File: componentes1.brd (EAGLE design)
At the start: 160 x 100 mm, 14 parts, among them IC1 LD117AS33TR, K1 CQ1-12V, T1 BC337, U1 DS1307Z, X1 32.768KHZ

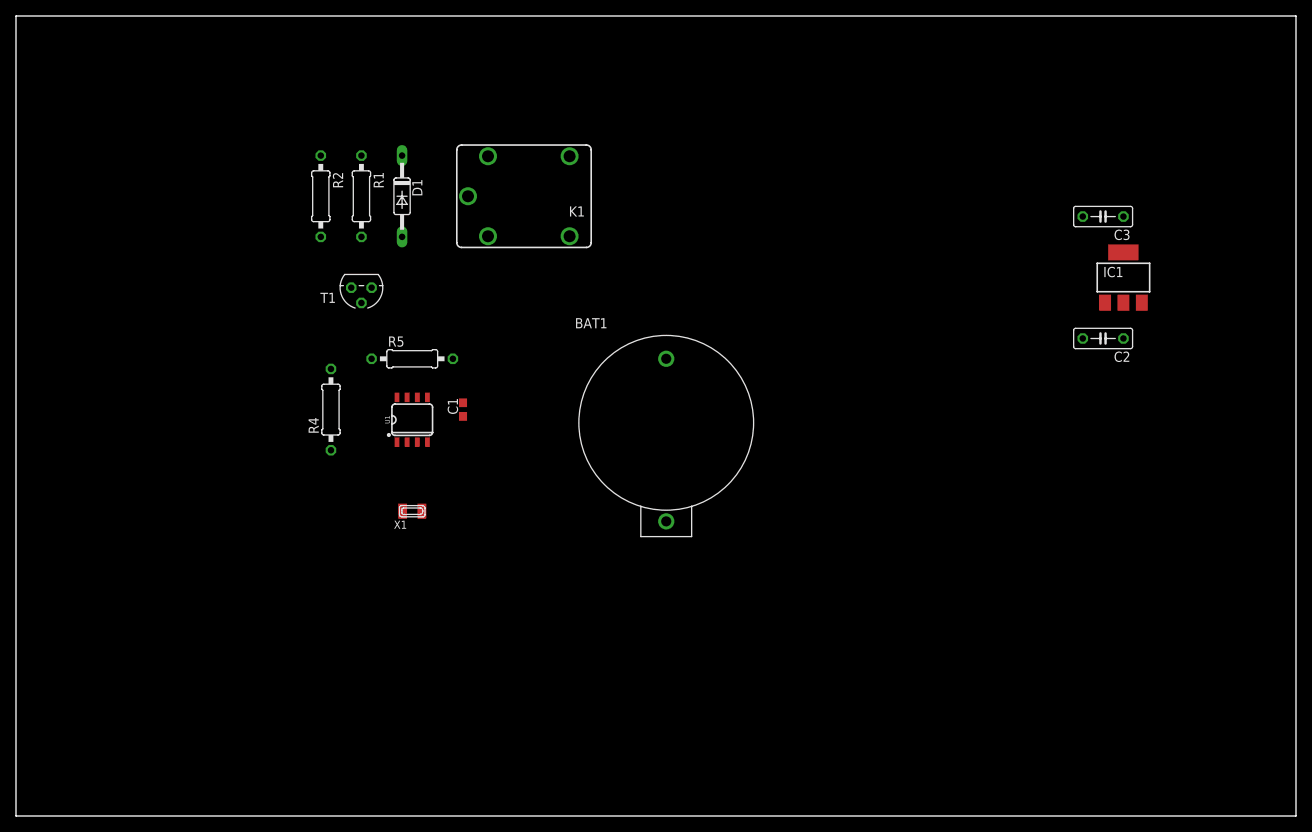
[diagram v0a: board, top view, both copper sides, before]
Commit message: se agrega board
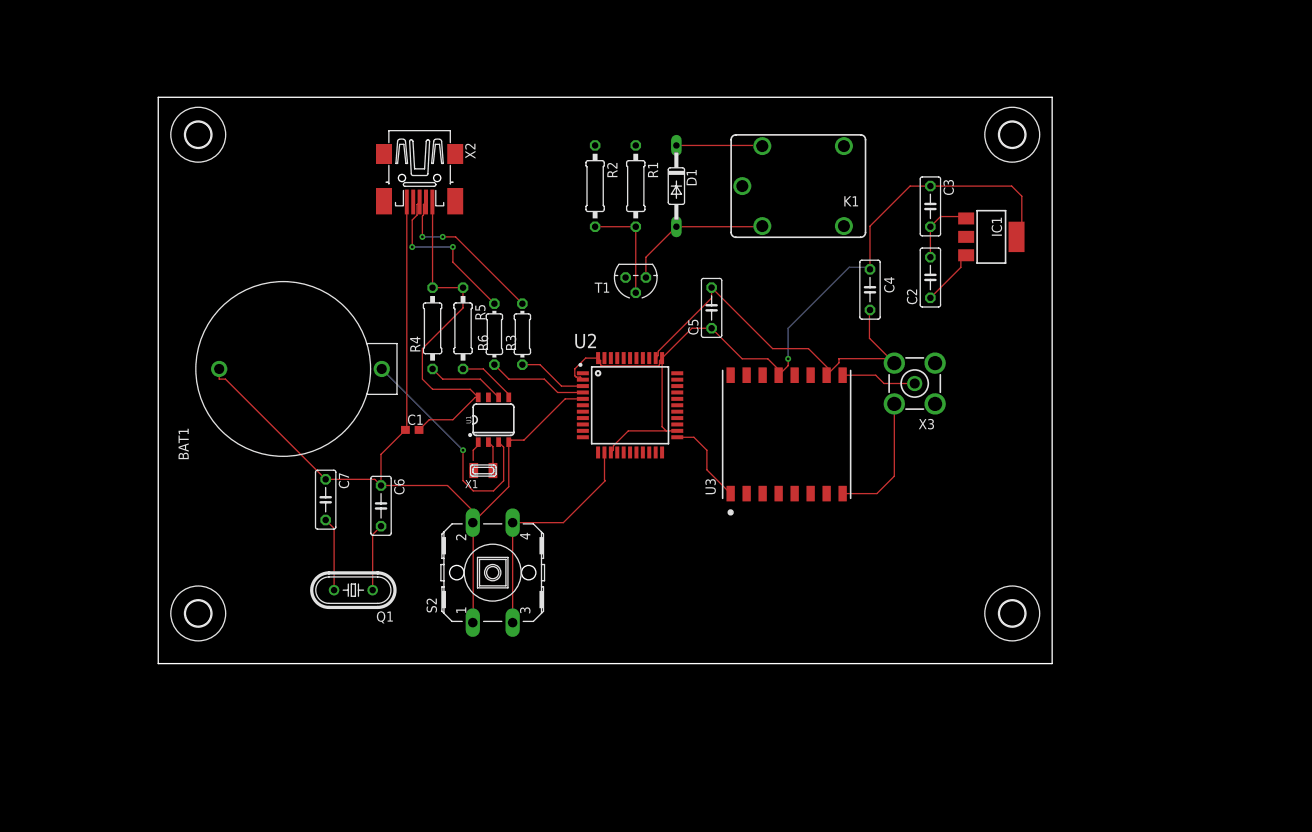
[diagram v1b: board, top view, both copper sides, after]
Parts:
- added C4, C5, C6, C7: (no value), rcl:C050-025X075
- added H1, H2, H3, H4: MOUNT-HOLE3.2, holes:3,2
- added Q1: (no value), crystal:HC49/S
- added R3, R6: (no value), rcl:0204/7
- added S2: (no value), switch-omron:B3F-40XX
- added U2: ATMEGA32U4-AU, ATMEGA32U4-AU:QFP80P1200X1200X120-44N
- added U3: RFM95W-868S2, RFM95W-868S2:XCVR_RFM95W-868S2
- added X2: MINI-USB-32005-201, con-cypressindustries:32005-201
- added X3: BU-SMA-V, con-coax:BU-SMA-V
- moved BAT1 40.3 mm to (45.7, 55.9), turned to 90 degrees
- moved K1 34.3 mm to (97.8, 78.7)
- moved D1 34.3 mm to (82.5, 78.7)
- moved R1 34.3 mm to (77.5, 78.7)
- moved R2 34.3 mm to (72.4, 78.7)
- moved T1 34.3 mm to (77.5, 67.3)
- moved C2 22.9 mm to (114.3, 67.3), turned to 90 degrees
- moved C3 21.6 mm to (114.3, 76.2), turned to 270 degrees
- moved IC1 17.3 mm to (121.9, 72.4), turned to 270 degrees
- moved R4 16.3 mm to (52.1, 61.0)
- moved X1 10.2 mm to (58.4, 43.2)
- moved U1 10.2 mm to (59.7, 49.5)
- moved R5 7.41 mm to (55.9, 61.0), turned to 270 degrees
- moved C1 6.84 mm to (49.5, 48.3), turned to 0 degrees
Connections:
- new net ANT: U3.9, X3.1
- new net ID: X2.4
- new net N$10: U2.42
- new net N$11: U2.17
- new net N$12: U2.8
- new net N$13: U2.9
- new net N$14: U2.10
- new net N$15: U2.11
- new net N$16: U2.28
- new net N$17: U2.29
- new net N$18: U2.30
- new net N$19: U2.12
- new net N$20: U2.18
- new net N$21: U2.19
- new net N$22: U2.20
- new net N$23: U2.21
- new net N$24: U2.25
- new net N$25: U2.22
- new net N$26: U2.26
- new net N$27: U2.27
- new net N$28: U2.6
- new net N$29: R3.1, U2.3
- new net N$30: U2.36
- new net N$31: U2.37
- new net N$32: U2.38
- new net N$33: U2.39
- new net N$34: U2.40
- new net N$35: U2.41
- new net N$36: U2.1
- new net N$37: U2.32
- new net N$38: U2.31
- new net N$39: U2.16
- new net N$40: R3.2, X2.2
- new net N$41: U3.6
- new net N$42: R6.2, X2.3
- new net N$43: R6.1, U2.4
- new net N$44: U2.33
- new net N$45: U3.2
- new net N$46: U3.4
- new net N$47: U3.5
- new net N$49: U3.7
- new net N$50: U3.11
- new net N$51: U3.12
- new net N$52: U3.14
- new net N$53: U3.15
- new net N$54: U3.16
- new net N$58: U3.3
- new net N$8: U2.7
- new net RESET: S2.3, S2.4, U2.13
- new net XTAL1: C6.2, Q1.1
- new net XTAL2: C7.2, Q1.2
- net 3.3V: now also C4.1, C5.1, U2.14, U2.2, U2.24, U2.34, U2.44, U3.13
- net GND: now also C4.2, C5.2, C6.1, C7.1, S2.1, S2.2, U2.15, U2.23, U2.35, U2.43, U2.5, U3.1, U3.10, U3.8, X2.5, X3.2, X3.3, X3.4, X3.5
- net VCC: now also X2.1
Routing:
- net GND: track 0.00 -> 189.6 mm
- net 3.3V: track 0.00 -> 102.8 mm, vias 0 -> 1
- net VCC: track 0.00 -> 44.5 mm
- net RESET: track 0.00 -> 29.8 mm
- net N$4: track 0.00 -> 29.4 mm, vias 0 -> 1
- net N$40: track 0.00 -> 20.5 mm, vias 0 -> 2
- net N$42: track 0.00 -> 20.3 mm, vias 0 -> 2
- net N$3: track 0.00 -> 18.1 mm
- net N$6: track 0.00 -> 13.3 mm
- net N$43: track 0.00 -> 12.5 mm
- net SCL: track 0.00 -> 9.73 mm
- net N$5: track 0.00 -> 9.55 mm
- net ANT: track 0.00 -> 9.44 mm
- net XTAL2: track 0.00 -> 9.20 mm
- net N$29: track 0.00 -> 8.67 mm
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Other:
- board size 160 x 100 mm -> 111.7 x 70.8 mm
